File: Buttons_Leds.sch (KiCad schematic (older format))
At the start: 41 parts, among them P3 CONN_02X02, P4 CONN_01X02, Q2 2N7002, Q3 2N7002, Q4 2N7002, Q5 2N7002, SW1 TEC_1, SW2 TEC_1, SW3 TEC_1, SW4 TEC_1, U3 LM317_SOT223

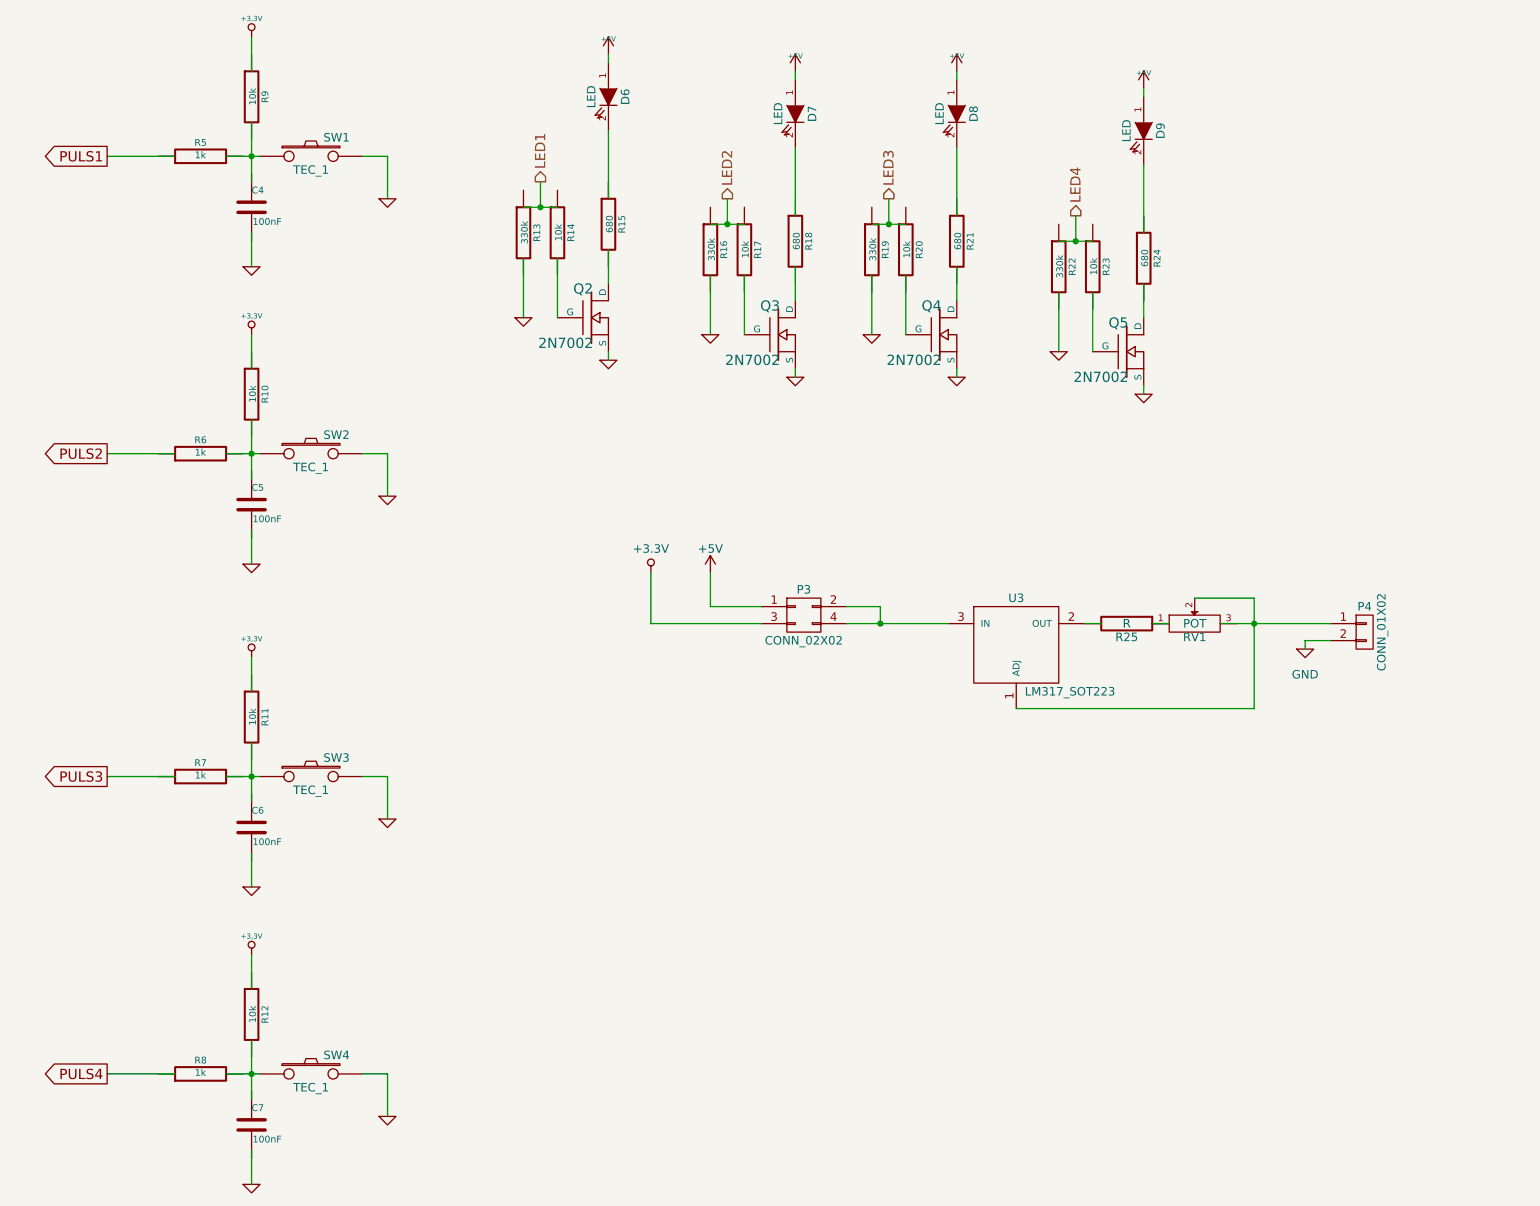
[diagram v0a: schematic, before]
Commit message: Arreglo Max3232_ok, Fuente_ok, Buttons&Leds, OK.Fuente correinte OK, Potenciometros OK y LM35 OK.
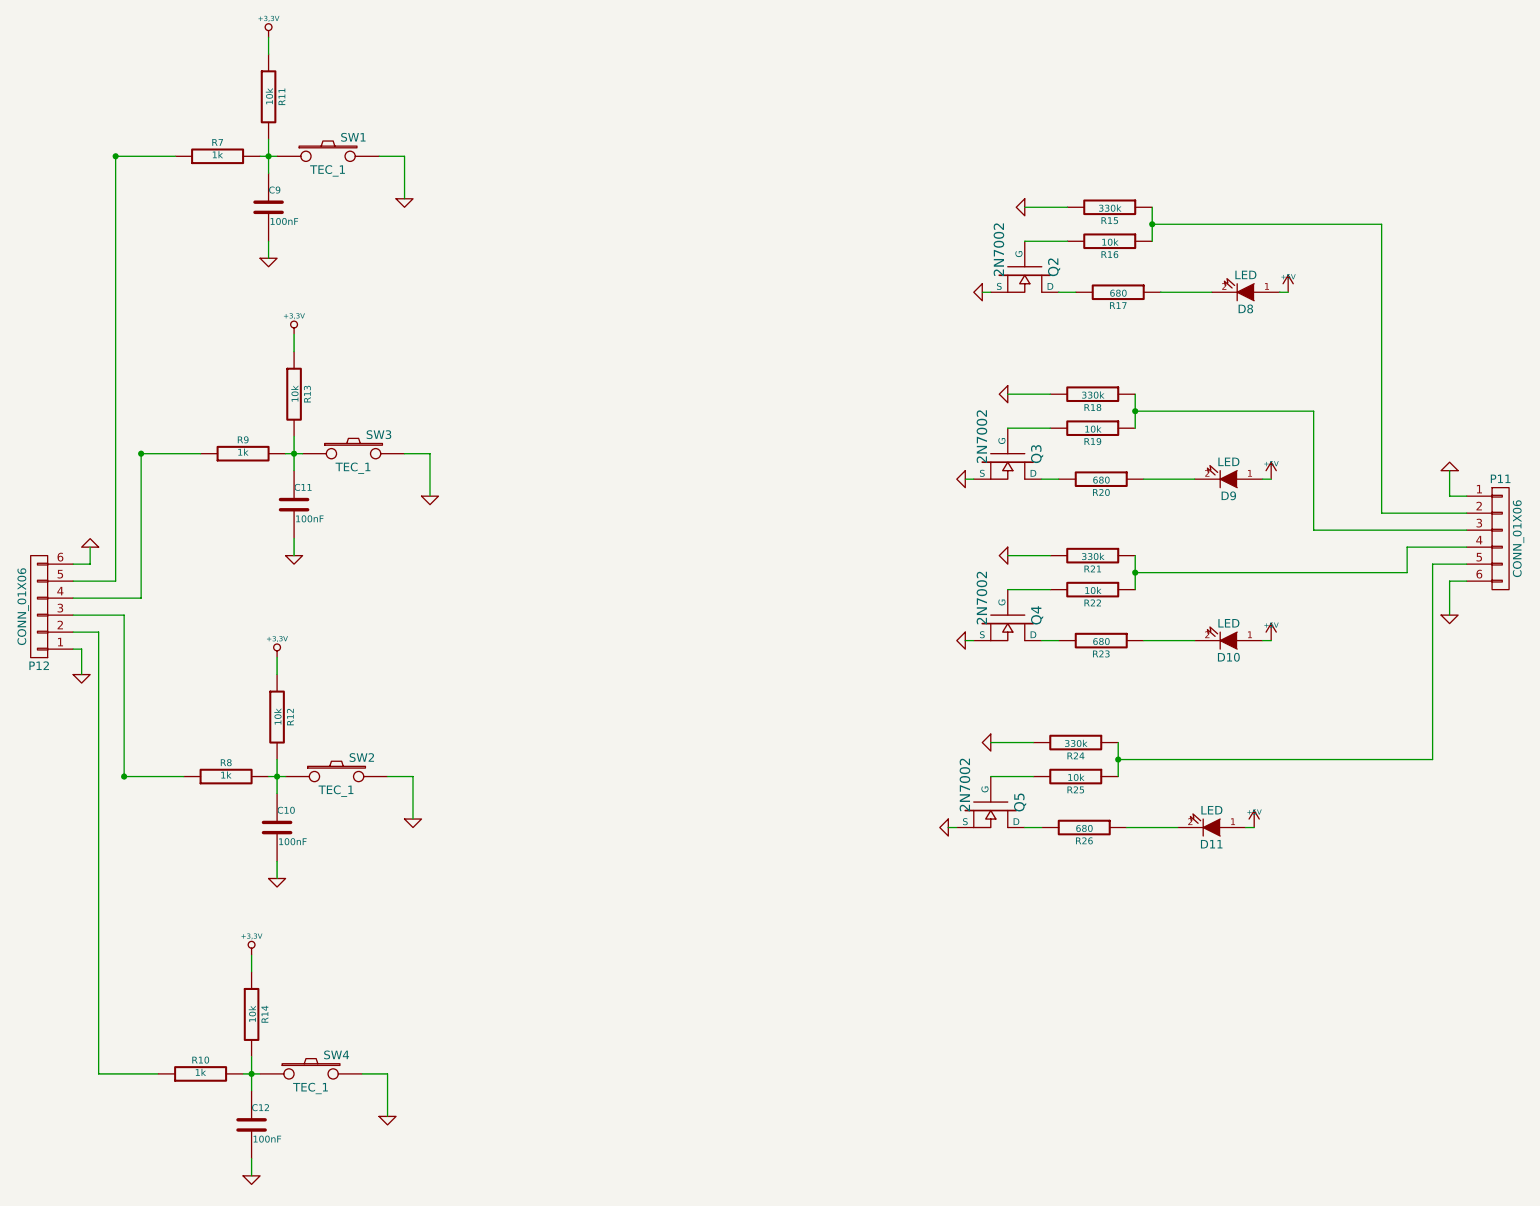
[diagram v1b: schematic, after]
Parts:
- removed C4, C5, C6: 100nF, c_0805, symbol C
- removed D8: LED, LED-0805, symbol LED
- removed P3: CONN_02X02, symbol CONN_02X02
- removed P4: CONN_01X02, symbol CONN_01X02
- removed R14, R17, R20: 10k, SM0805, symbol R
- removed R25: R, symbol R
- removed R5, R6: 1k, SM0805, symbol R
- removed RV1: POT, symbol POT
- removed U3: LM317_SOT223, symbol LM317_SOT223
- added C10, C11, C9: 100nF, c_0805, symbol C
- added D10: LED, LED-0805, symbol LED
- added P11, P12: CONN_01X06, symbol CONN_01X06
- added R12, R16, R22: 10k, SM0805, symbol R
- added R15: 330k, SM0805, symbol R
- added R23: 680, SM0805, symbol R
- R10, R9: value 10k -> 1k; Descripción RES 10K OHM 1/8W 5% 0805 SMD -> RES 1K OHM 1/8W 5% 0805 SMD; Digikey P10KACT-ND -> 311-1.0KARCT-ND; Fabricante Panasonic Electronic Components -> Yageo; Nro de parte ERJ-6GEYJ103V -> RC0805JR-071KL
- R13, R19: value 330k -> 10k; Descripción RES 330K OHM 1/8W 5% 0805 -> RES 10K OHM 1/8W 5% 0805 SMD; Digikey RMCF0805JT330KCT-ND -> P10KACT-ND; Fabricante Stackpole Electronics Inc -> Panasonic Electronic Components; Nro de parte RMCF0805JT330K -> ERJ-6GEYJ103V
- R21: value 680 -> 330k; Descripción RES 680 OHM 1/10W .5% 0805 SMD -> RES 330K OHM 1/8W 5% 0805; Digikey RR12P680DCT-ND -> RMCF0805JT330KCT-ND; Fabricante Susumu -> Stackpole Electronics Inc; Nro de parte RR1220P-681-D -> RMCF0805JT330K
- renumbered C7 to C12, D9 to D11, D6 to D8, D7 to D9, R12 to R14, R15 to R17, R16 to R18, R18 to R20, R22 to R24, R23 to R25, R24 to R26
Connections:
- net labels removed: +3.3V, LED1, LED2, LED3, LED4, PULS1, PULS2, PULS3, PULS4
- wire segments 75 -> 84
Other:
- moved on the sheet: D11, D8, D9, Q2, Q4, R17, R18, R20, R24, R25, R26
